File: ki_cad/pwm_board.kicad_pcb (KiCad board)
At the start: 4 copper layers, 51 x 41 mm, 87 parts, among them J0 Conn_01x03_Pin, J1 Conn_01x03_Pin, J10 Conn_01x04_Pin, J11 SWD_CONN, J12 Conn_01x02_Pin, J13 Conn_01x02_Pin, J14 Conn_01x02_Pin, J15 Conn_01x02_Pin, J16 Conn_01x02_Pin, J17 Conn_01x02_Pin, J2 Conn_01x03_Pin, J3 Conn_01x03_Pin, J4 Conn_01x03_Pin, J5 Conn_01x03_Pin, J6 Conn_01x03_Pin, J7 Conn_01x03_Pin, J8 Conn_01x03_Pin, J9 Conn_01x03_Pin, Q0 Q_NMOS, Q1 Q_NMOS, Q2 Q_NMOS, Q3 Q_NMOS, Q4 Q_NMOS, Q5 Q_NMOS, Q6 Q_NMOS, SW1 USER_SW, U1 STM32L010F4P6, U2 SP3485EN, U3 SY81051, U4 PCA9685PW

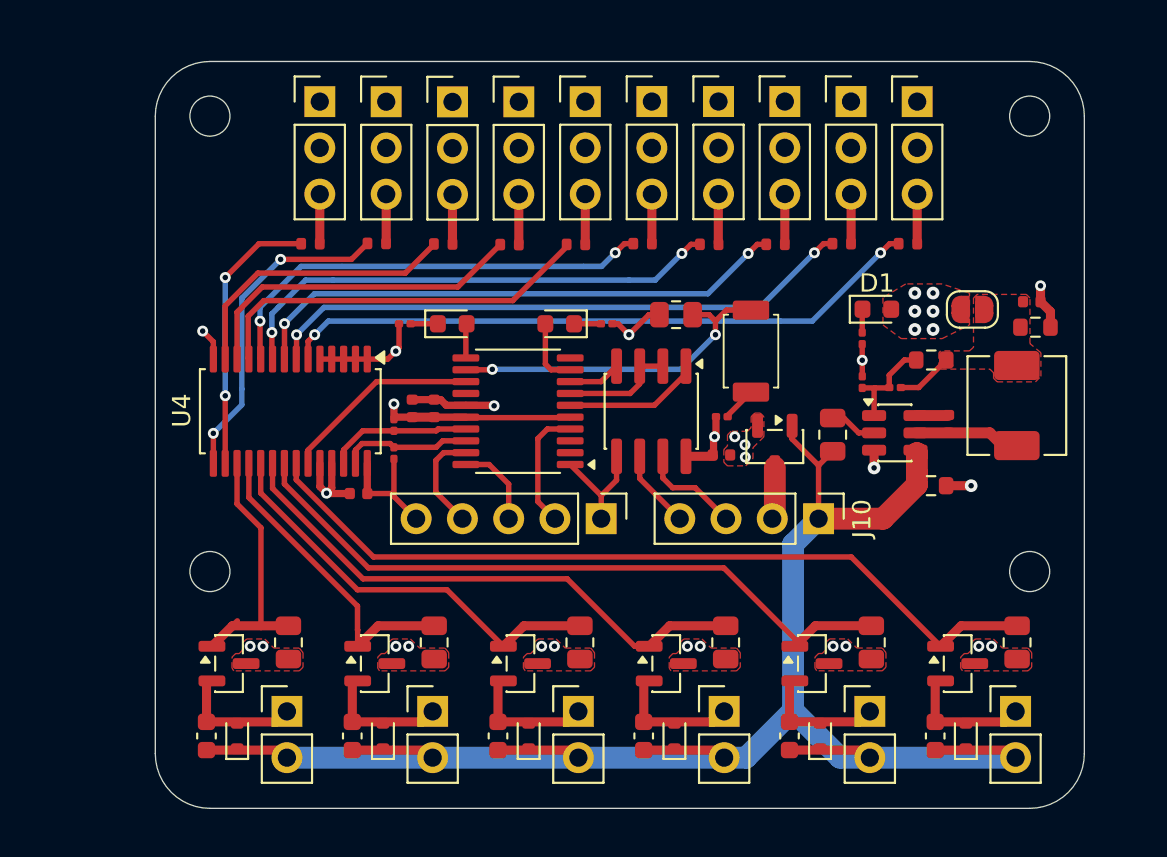
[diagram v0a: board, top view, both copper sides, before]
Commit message: update after feedback (purchased)
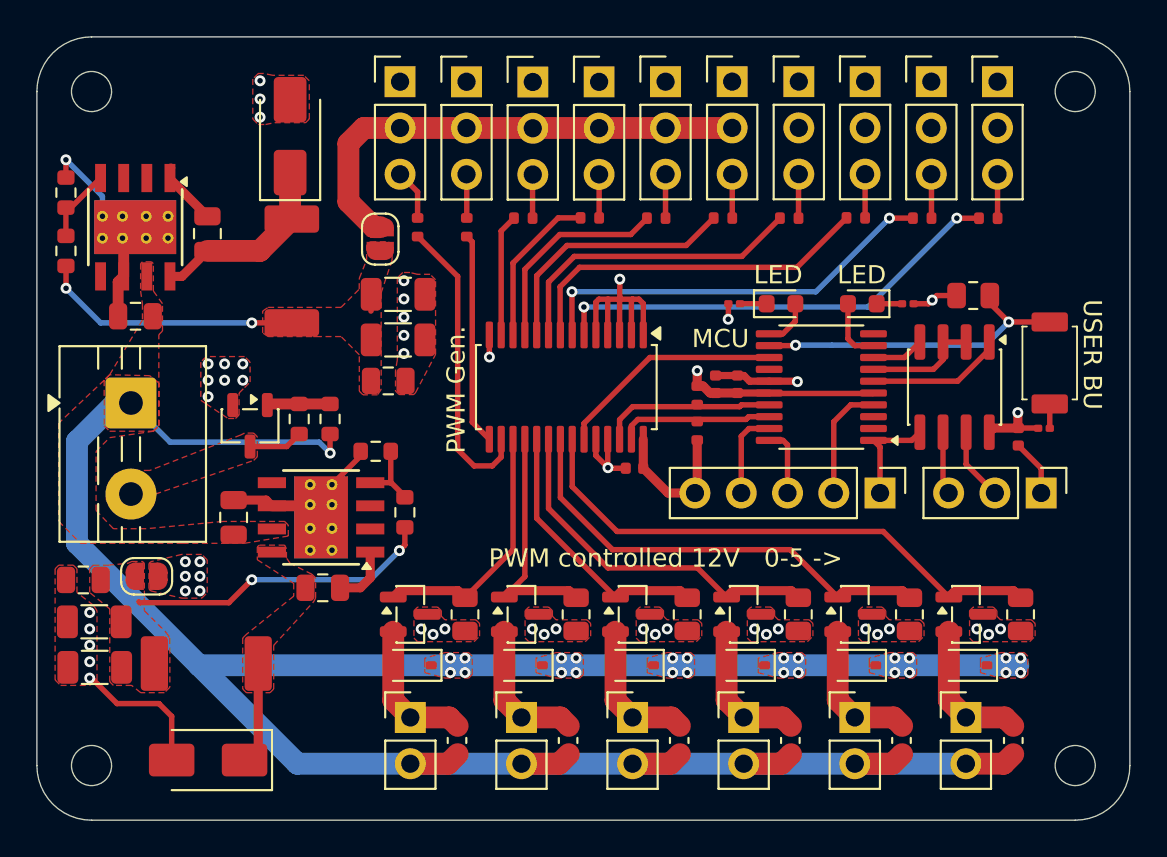
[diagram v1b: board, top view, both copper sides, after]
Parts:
- removed C13: 10u, Capacitor_SMD:C_0402_1005Metric
- removed J10: Conn_01x04_Pin, Connector_PinHeader_2.54mm:PinHeader_1x04_P2.54mm_Vertical
- removed Q6: Q_NMOS, Custom:SOT-23-3
- removed U4: PCA9685PW, Package_SO:TSSOP-28_4.4x9.7mm_P0.65mm
- added C16: 10u, Capacitor_SMD:C_0805_2012Metric, F.Cu at (80.3, 51.7)
- added C17: 10n, Capacitor_SMD:C_0805_2012Metric, F.Cu at (84.3, 47.1)
- added C18: 100u, Capacitor_SMD:C_1206_3216Metric, F.Cu at (78.0, 68.5)
- added C19: 100u, Capacitor_SMD:C_1206_3216Metric, F.Cu at (78.1, 71.0)
- added C20: 22u, Capacitor_SMD:C_0805_2012Metric, F.Cu at (77.5, 66.2)
- added C21: 10u, Capacitor_SMD:C_0402_1005Metric, F.Cu at (107.7, 60.0)
- added D10: SS34, Diode_SMD:D_SMA, F.Cu at (88.8, 41.8)
- added J18: Communiation_IN, Connector_PinHeader_2.54mm:PinHeader_1x03_P2.54mm_Vertical, F.Cu at (130.0, 61.4)
- added J19: Power_IN, TerminalBlock:TerminalBlock_MaiXu_MX126-5.0-02P_1x02_P5.00mm, F.Cu at (80.1, 56.4)
- added JP2: SolderJumper_Open, Jumper:SolderJumper-2_P1.3mm_Open_RoundedPad1.0x1.5mm, F.Cu at (93.8, 47.5)
- added L2: 15u, Custom:CYA0630, F.Cu at (88.9, 49.2)
- added Q7: Q_NMOS, Custom:SOT-23-3, F.Cu at (86.6, 57.7)
- added R28: 6K8, Resistor_SMD:R_0603_1608Metric, F.Cu at (76.5, 44.9)
- added R9: 12k, Resistor_SMD:R_0603_1608Metric, F.Cu at (76.5, 48.1)
- added U5: PCA9635PW,118, Package_SO:TSSOP-28_4.4x9.7mm_P0.65mm, F.Cu at (104.0, 55.6)
- added U6: TPS5430DDA, Package_SO:TI_SO-PowerPAD-8_ThermalVias, F.Cu at (80.3, 46.8)
- C10: value 100p -> 22u; footprint Resistor_SMD:R_0603_1608Metric -> Capacitor_SMD:C_0805_2012Metric
- C11: value 22u -> 10u; footprint Resistor_SMD:R_0603_1608Metric -> Capacitor_SMD:C_0805_2012Metric
- C12: value 10u -> 10n; footprint Capacitor_SMD:C_0402_1005Metric -> Capacitor_SMD:C_0805_2012Metric
- C8: value 22u -> 100u; footprint Resistor_SMD:R_0603_1608Metric -> Capacitor_SMD:C_1206_3216Metric
- C9: value 100n -> 100u; footprint Capacitor_SMD:C_0402_1005Metric -> Capacitor_SMD:C_1206_3216Metric
- D1: value RED -> SS34; footprint Diode_SMD:D_0603_1608Metric -> Diode_SMD:D_SMA
- D4, D5, D6, D7, D8, D9: footprint Diode_SMD:D_SOD-523 -> Diode_SMD:D_SOD-323
- JP1: value SolderJumper_2_Open -> SolderJumper_Open
- L1: value 3u3 -> 15u; footprint Inductor_SMD:L_KOHERelec_MDA5030 -> Custom:CYA0630
- R20, R21: footprint Resistor_SMD:R_0201_0603Metric -> Resistor_SMD:R_0402_1005Metric
- R5: value 10K -> 12k; footprint Resistor_SMD:R_0805_2012Metric -> Resistor_SMD:R_0603_1608Metric
- R6: value 82k -> 6K8; footprint Resistor_SMD:R_0201_0603Metric -> Resistor_SMD:R_0603_1608Metric
- R7: value 18k -> 51k; footprint Resistor_SMD:R_0201_0603Metric -> Resistor_SMD:R_0603_1608Metric
- R8: value 1K5 -> 51k; footprint Resistor_SMD:R_0201_0603Metric -> Resistor_SMD:R_0603_1608Metric
- U3: value SY81051 -> TPS5430DDA; footprint Package_TO_SOT_SMD:TSOT-23-6 -> Package_SO:TI_SO-PowerPAD-8_ThermalVias
- moved JP1 47.6 mm to (80.9, 66.0), turned to 0 degrees
- moved L1 46.7 mm to (84.2, 70.8), turned to 180 degrees
- moved C11 45.2 mm to (85.7, 62.7), turned to 90 degrees
- moved D1 44.3 mm to (84.3, 76.0), turned to 180 degrees
- moved C12 42.0 mm to (90.6, 66.6), turned to 180 degrees
- moved H2 35.7 mm to (131.9, 76.3)
- moved U3 31.8 mm to (90.5, 62.7), turned to 180 degrees
- moved R8 31.2 mm to (89.3, 57.3), turned to -90 degrees
- moved C8 31.1 mm to (94.7, 50.5)
- moved C9 30.6 mm to (94.7, 53.0), turned to 0 degrees
- moved C10 29.8 mm to (94.2, 55.2), turned to 0 degrees
- moved R7 29.3 mm to (91.0, 57.3)
- moved R6 28.7 mm to (93.5, 59.1)
- moved H4 26.5 mm to (131.9, 39.4)
- moved R5 23.9 mm to (95.1, 62.5)
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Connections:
- C10 pad 1: +3V3 -> Net-(JP2-A)
- C10 pad 2: Net-(U3-FB) -> GND
- C11 pad 1: +3V3 -> +12V
- C12 pad 1: +3V3 -> Net-(U3-BOOT)
- C12 pad 2: GND -> Net-(D1-K)
- C8 pad 1: +12V -> Net-(JP2-A)
- C9 pad 1: Net-(U3-BS) -> Net-(JP2-A)
- C9 pad 2: Net-(U3-LX) -> GND
- D1 pad 2: +3V3 -> GND
- J4 pad 2: +3V3 -> +3V3_1
- J5 pad 2: +3V3 -> +3V3_1
- J6 pad 2: +3V3 -> +3V3_1
- J7 pad 2: +3V3 -> +3V3_1
- J8 pad 2: +3V3 -> +3V3_1
- J9 pad 2: +3V3 -> +3V3_1
- JP1 pad 1: +3V3 -> Net-(JP1-A)
- L1 pad 1: Net-(U3-LX) -> Net-(D1-K)
- L1 pad 2: +3V3 -> Net-(JP1-A)
- R5 pad 1: +12V -> Net-(JP1-A)
- R5 pad 2: Net-(U3-EN) -> Net-(U3-VSENSE)
- R6 pad 1: +3V3 -> Net-(U3-VSENSE)
- R6 pad 2: Net-(U3-FB) -> GND
- R7 pad 1: Net-(U3-FB) -> +12V
- R7 pad 2: GND -> Net-(Q7-PadG)
- R8 pad 1: GND -> Net-(Q7-PadG)
- R8 pad 2: Net-(D1-K) -> /power/GND_IN
- U3 pad 1: Net-(U3-FB) -> Net-(U3-BOOT)
- U3 pad 2: Net-(U3-EN) -> unconnected-(U3-NC-Pad2)
- U3 pad 3: GND -> unconnected-(U3-NC-Pad3)
- U3 pad 4: +12V -> Net-(U3-VSENSE)
- U3 pad 5: Net-(U3-LX) -> unconnected-(U3-EN-Pad5)
- U3 pad 6: Net-(U3-BS) -> GND
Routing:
- net +12V: track 95.6 -> 138.3 mm, vias 0 -> 25
- net +3V3_1: track 0.00 -> 27.0 mm
- net GND: track 36.1 -> 62.4 mm, vias 24 -> 45
- net Net-(JP1-A): track 0.00 -> 17.1 mm, vias 0 -> 2
- net /pwm/MOTOR_PWM_5: track 44.7 -> 30.0 mm
- net Net-(JP2-A): track 0.00 -> 14.6 mm, vias 0 -> 2
- net /pwm/MOTOR_PWM_4: track 37.6 -> 24.9 mm
- net Net-(D10-K): track 0.00 -> 10.8 mm
- net /pwm/SERVO_PWM_4: track 24.8 -> 14.3 mm, vias 2 -> 0
- net /pwm/SERVO_PWM_3: track 27.6 -> 17.1 mm, vias 2 -> 0
- net /pwm/MOTOR_PWM_3: track 30.3 -> 19.8 mm
- net /pwm/SERVO_PWM_0: track 35.6 -> 25.2 mm
- net /pwm/SERVO_PWM_2: track 30.2 -> 19.9 mm, vias 2 -> 0
- net /pwm/SERVO_PWM_5: track 21.6 -> 11.5 mm
- net /pwm/SERVO_PWM_1: track 32.8 -> 22.8 mm
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- added copper zone on F.Cu, net +12V
- added copper zone on F.Cu, net /power/GND_IN
- added copper zone on F.Cu, net Net-(D1-K)
- added copper zone on F.Cu, net Net-(JP1-A)
- added copper zone on F.Cu, net Net-(JP2-A)
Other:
- board size 51 x 41 mm -> 60 x 43 mm
- board text added: "LED"
- board text added: "MCU"
- board text added: "PWM Gen."
- board text added: "PWM controlled 12V 0-5 ->"
- board text added: "RS A"
- board text added: "RS B"
- board text added: "USER BU"
- board text removed: "12V"
- board text removed: "RS-485 A"
- board text removed: "RS-485 B"
